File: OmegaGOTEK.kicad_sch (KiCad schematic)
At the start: 75 parts, among them J3 Conn_01x02_Pin, J4 Conn_01x04_Pin, J5 Conn_01x02_Pin, J7 Conn_02x03_Counter_Clockwise, M0 Conn_01x02_Pin, P1 FLOPPY CONNECTOR, P2 PWR, P3 USB_A, Q1 MOFSET N DGS, Q2 MOFSET N DGS, Q3 MOFSET N DGS, Q4 MOFSET N DGS, Q5 MOFSET N DGS, Q6 MOFSET N DGS, U1 74HC04, U3 AT32F435RGT7, U4 AMS1117-3.3, U5 TM1651, U8 GD5F1GQ4UFYIGR, Y1 8 MHz

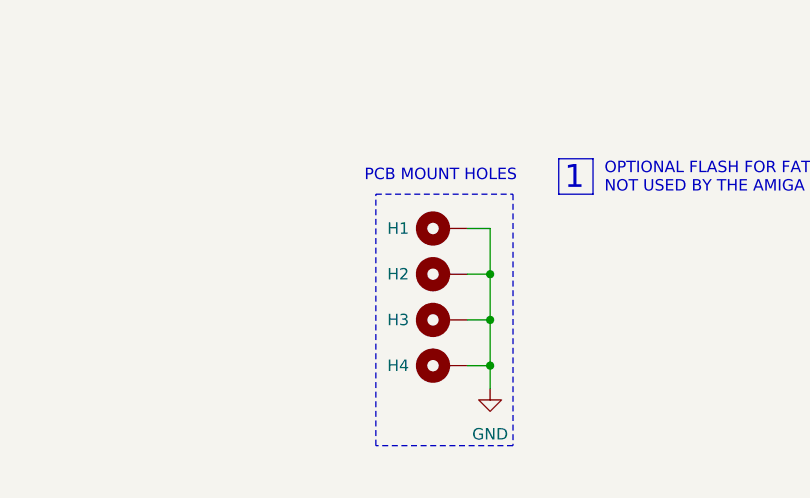
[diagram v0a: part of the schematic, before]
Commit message: More board work
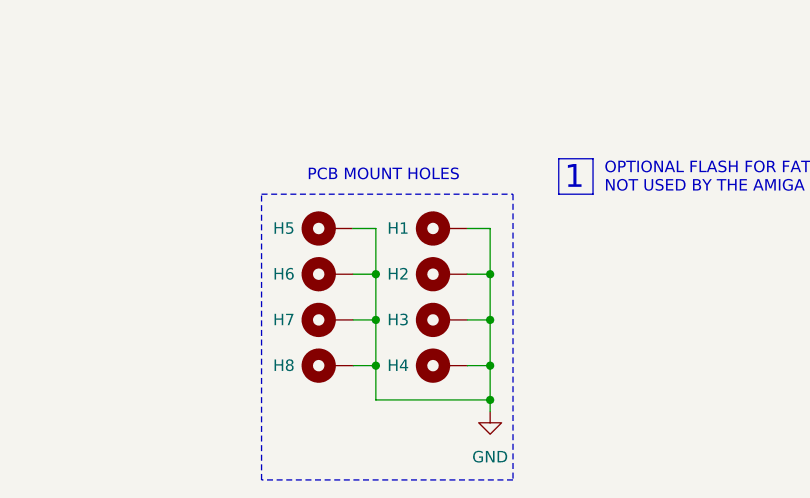
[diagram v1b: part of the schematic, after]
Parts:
- added H5, H6, H7, H8: MountingHole, MountingHole:MountingHole_2.2mm_M2_Pad_Via, symbol Mechanical:MountingHole_Pad
- C1: footprint Capacitor_SMD:C_0805_2012Metric_Pad1.18x1.45mm_HandSolder -> Capacitor_THT:CP_Radial_D5.0mm_P2.50mm
- Y1: footprint Crystal:Crystal_HC49-U_Vertical -> Crystal:Crystal_HC49-4H_Vertical
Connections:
- net GND: now also H5.1, H6.1, H7.1, H8.1
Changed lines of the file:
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@@
   (junction (at 242.57 304.8) (diameter 0) (color 0 0 0 0)
   )
+  (junction (at 466.09 397.51) (diameter 0) (color 0 0 0 0)
+  )
   (junction (at 214.63 135.89) (diameter 0) (color 0 0 0 0)
   )
@@
   (junction (at 278.13 163.83) (diameter 0) (color 0 0 0 0)
   )
+  (junction (at 453.39 388.62) (diameter 0) (color 0 0 0 0)
+  )
   (junction (at 427.99 168.91) (diameter 0) (color 0 0 0 0)
   )
@@
   (junction (at 90.17 325.12) (diameter 0) (color 0 0 0 0)
   )
+  (junction (at 453.39 383.54) (diameter 0) (color 0 0 0 0)
+  )
   (junction (at 427.99 273.05) (diameter 0) (color 0 0 0 0)
   )
@@
   (junction (at 382.27 299.72) (diameter 0) (color 0 0 0 0)
   )
+  (junction (at 453.39 393.7) (diameter 0) (color 0 0 0 0)
+  )
   (junction (at 346.71 146.05) (diameter 0) (color 0 0 0 0)
   )
@@
     (stroke (width 0) (type default))
   )
+  (wire (pts (xy 466.09 397.51) (xy 466.09 398.78))
+    (stroke (width 0) (type default))
+  )
   (wire (pts (xy 144.78 72.39) (xy 144.78 69.85))
     (stroke (width 0) (type default))
@@
     (stroke (width 0) (type default))
   )
+  (wire (pts (xy 453.39 378.46) (xy 453.39 383.54))
+    (stroke (width 0) (type default))
+  )
   (wire (pts (xy 99.06 349.25) (xy 196.85 349.25))
     (stroke (width 0) (type default))
@@
     (stroke (width 0) (type default))
   )
+  (wire (pts (xy 450.85 383.54) (xy 453.39 383.54))
+    (stroke (width 0) (type default))
+  )
   (wire (pts (xy 424.18 97.79) (xy 431.8 97.79))
     (stroke (width 0) (type default))
@@
     (stroke (width 0) (type default))
   )
+  (wire (pts (xy 453.39 397.51) (xy 466.09 397.51))
+    (stroke (width 0) (type default))
+  )
   (wire (pts (xy 273.05 312.42) (xy 273.05 320.04))
     (stroke (width 0) (type default))
@@
     (stroke (width 0) (type default))
   )
+  (wire (pts (xy 450.85 393.7) (xy 453.39 393.7))
+    (stroke (width 0) (type default))
+  )
   (wire (pts (xy 498.475 231.14) (xy 498.475 213.36))
     (stroke (width 0) (type default))
@@
     (stroke (width 0) (type default))
   )
-  (wire (pts (xy 466.09 393.7) (xy 466.09 396.24))
-    (stroke (width 0) (type default))
-  )
   (wire (pts (xy 382.905 224.79) (xy 380.365 224.79))
     (stroke (width 0) (type default))
@@
     (stroke (width 0) (type default))
   )
+  (wire (pts (xy 450.85 378.46) (xy 453.39 378.46))
+    (stroke (width 0) (type default))
+  )
   (wire (pts (xy 400.05 146.05) (xy 400.05 140.97))
     (stroke (width 0) (type default))
@@
     (stroke (width 0) (type default))
   )
+  (wire (pts (xy 453.39 388.62) (xy 453.39 393.7))
+    (stroke (width 0) (type default))
+  )
   (wire (pts (xy 196.85 349.25) (xy 196.85 314.96))
     (stroke (width 0) (type default))
@@
     (stroke (width 0) (type default))
   )
+  (wire (pts (xy 453.39 383.54) (xy 453.39 388.62))
+    (stroke (width 0) (type default))
+  )
   (wire (pts (xy 471.805 228.6) (xy 474.98 228.6))
     (stroke (width 0) (type default))
@@
     (stroke (width 0) (type default))
   )
+  (wire (pts (xy 466.09 393.7) (xy 466.09 397.51))
+    (stroke (width 0) (type default))
+  )
   (wire (pts (xy 427.99 171.45) (xy 431.8 171.45))
     (stroke (width 0) (type default))
@@
     (stroke (width 0) (type default))
   )
+  (wire (pts (xy 453.39 393.7) (xy 453.39 397.51))
+    (stroke (width 0) (type default))
+  )
   (wire (pts (xy 427.99 173.99) (xy 363.22 173.99))
     (stroke (width 0) (type default))
@@
     (stroke (width 0) (type default))
   )
+  (wire (pts (xy 450.85 388.62) (xy 453.39 388.62))
+    (stroke (width 0) (type default))
+  )
   (wire (pts (xy 102.87 327.66) (xy 91.44 327.66))
     (stroke (width 0) (type default))
@@
     (stroke (width 0) (type default))
   )
-  (rectangle (start 453.39 374.65) (end 468.63 402.59)
+  (rectangle (start 440.69 374.65) (end 468.63 406.4)
     (stroke (width 0) (type dash))
     (fill (type none))
@@
     (effects (font (size 1.27 1.27)) (justify left bottom))
   )
-  (text "PCB MOUNT HOLES" (at 452.12 373.38 0)
+  (text "PCB MOUNT HOLES" (at 445.77 373.38 0)
     (effects (font (size 1.27 1.27)) (justify left bottom))
   )
@@
     )
   )
+  (symbol (lib_id "Mechanical:MountingHole_Pad") (at 448.31 393.7 90) (unit 1)
+    (in_bom yes) (on_board yes) (dnp no)
+    (property "Reference" "H8" (at 441.96 393.7 90)
+      (effects (font (size 1.27 1.27)) (justify right))
+    )
+    (property "Value" "MountingHole" (at 447.04 391.16 0)
+      (effects (font (size 1.27 1.27)) (justify left) hide)
+    )
+    (property "Footprint" "MountingHole:MountingHole_2.2mm_M2_Pad_Via" (at 448.31 393.7 0)
+      (effects (font (size 1.27 1.27)) hide)
+    )
+    (property "Datasheet" "~" (at 448.31 393.7 0)
+      (effects (font (size 1.27 1.27)) hide)
+    )
+    (pin "1")
+    (instances
+      (project "OmegaGOTEK"
+        (path "/1fd3d41e-a7ac-473b-adfc-4c72d1e05d19"
+          (reference "H8") (unit 1)
+        )
+      )
+    )
+  )
   (symbol (lib_id "Device:Q_NMOS_DGS") (at 142.24 264.16 0) (unit 1)
     (in_bom yes) (on_board yes) (dnp no) (fields_autoplaced)
@@
       (effects (font (size 1.27 1.27)) (justify right))
     )
-    (property "Footprint" "Crystal:Crystal_HC49-U_Vertical" (at 397.51 124.46 0)
+    (property "Footprint" "Crystal:Crystal_HC49-4H_Vertical" (at 397.51 124.46 0)
       (effects (font (size 1.27 1.27)) hide)
     )
@@
     )
   )
-  (symbol (lib_id "power:GND") (at 466.09 396.24 0) (unit 1)
+  (symbol (lib_id "power:GND") (at 466.09 398.78 0) (unit 1)
     (in_bom yes) (on_board yes) (dnp no) (fields_autoplaced)
-    (property "Reference" "#PWR034" (at 466.09 402.59 0)
+    (property "Reference" "#PWR034" (at 466.09 405.13 0)
       (effects (font (size 1.27 1.27)) hide)
     )
-    (property "Value" "GND" (at 466.09 401.32 0)
+    (property "Value" "GND" (at 466.09 403.86 0)
       (effects (font (size 1.27 1.27)))
     )
-    (property "Footprint" "" (at 466.09 396.24 0)
+    (property "Footprint" "" (at 466.09 398.78 0)
       (effects (font (size 1.27 1.27)) hide)
     )
-    (property "Datasheet" "" (at 466.09 396.24 0)
+    (property "Datasheet" "" (at 466.09 398.78 0)
       (effects (font (size 1.27 1.27)) hide)
     )
@@
     )
   )
+  (symbol (lib_id "Mechanical:MountingHole_Pad") (at 448.31 378.46 90) (unit 1)
+    (in_bom yes) (on_board yes) (dnp no)
+    (property "Reference" "H5" (at 441.96 378.46 90)
+      (effects (font (size 1.27 1.27)) (justify right))
+    )
+    (property "Value" "MountingHole" (at 447.04 375.92 0)
+      (effects (font (size 1.27 1.27)) (justify left) hide)
+    )
+    (property "Footprint" "MountingHole:MountingHole_2.2mm_M2_Pad_Via" (at 448.31 378.46 0)
+      (effects (font (size 1.27 1.27)) hide)
+    )
+    (property "Datasheet" "~" (at 448.31 378.46 0)
+      (effects (font (size 1.27 1.27)) hide)
+    )
+    (pin "1")
+    (instances
+      (project "OmegaGOTEK"
+        (path "/1fd3d41e-a7ac-473b-adfc-4c72d1e05d19"
+          (reference "H5") (unit 1)
+        )
+      )
+    )
+  )
   (symbol (lib_id "Device:R_US") (at 267.97 101.6 0) (unit 1)
     (in_bom yes) (on_board yes) (dnp no) (fields_autoplaced)
@@
     )
   )
+  (symbol (lib_id "Mechanical:MountingHole_Pad") (at 448.31 388.62 90) (unit 1)
+    (in_bom yes) (on_board yes) (dnp no)
+    (property "Reference" "H7" (at 441.96 388.62 90)
+      (effects (font (size 1.27 1.27)) (justify right))
+    )
+    (property "Value" "MountingHole" (at 447.04 386.08 0)
+      (effects (font (size 1.27 1.27)) (justify left) hide)
+    )
+    (property "Footprint" "MountingHole:MountingHole_2.2mm_M2_Pad_Via" (at 448.31 388.62 0)
+      (effects (font (size 1.27 1.27)) hide)
+    )
+    (property "Datasheet" "~" (at 448.31 388.62 0)
+      (effects (font (size 1.27 1.27)) hide)
+    )
+    (pin "1")
+    (instances
+      (project "OmegaGOTEK"
+        (path "/1fd3d41e-a7ac-473b-adfc-4c72d1e05d19"
+          (reference "H7") (unit 1)
+        )
+      )
+    )
+  )
   (symbol (lib_id "Device:R_US") (at 214.63 101.6 0) (unit 1)
     (in_bom yes) (on_board yes) (dnp no) (fields_autoplaced)
@@
     )
   )
+  (symbol (lib_id "Mechanical:MountingHole_Pad") (at 448.31 383.54 90) (unit 1)
+    (in_bom yes) (on_board yes) (dnp no)
+    (property "Reference" "H6" (at 441.96 383.54 90)
+      (effects (font (size 1.27 1.27)) (justify right))
+    )
+    (property "Value" "MountingHole" (at 447.04 381 0)
+      (effects (font (size 1.27 1.27)) (justify left) hide)
+    )
+    (property "Footprint" "MountingHole:MountingHole_2.2mm_M2_Pad_Via" (at 448.31 383.54 0)
+      (effects (font (size 1.27 1.27)) hide)
+    )
+    (property "Datasheet" "~" (at 448.31 383.54 0)
+      (effects (font (size 1.27 1.27)) hide)
+    )
+    (pin "1")
+    (instances
+      (project "OmegaGOTEK"
+        (path "/1fd3d41e-a7ac-473b-adfc-4c72d1e05d19"
+          (reference "H6") (unit 1)
+        )
+      )
+    )
+  )
   (symbol (lib_id "Switch:SW_Push") (at 369.57 102.87 0) (unit 1)
     (in_bom yes) (on_board yes) (dnp no)
@@
       (effects (font (size 1.27 1.27)) (justify left))
     )
-    (property "Footprint" "Capacitor_SMD:C_0805_2012Metric_Pad1.18x1.45mm_HandSolder" (at 336.2452 302.26 0)
+    (property "Footprint" "Capacitor_THT:CP_Radial_D5.0mm_P2.50mm" (at 336.2452 302.26 0)
       (effects (font (size 1.27 1.27)) hide)
     )
